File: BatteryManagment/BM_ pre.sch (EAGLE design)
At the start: 2 parts, among them U1 ATMEGA328P-AU

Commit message: Worked at the Schematic
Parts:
- added BATTERY+: Battery+, BM_pre:PAD
- added BATTERY-: PAD, BM_pre:PAD
- added C10, C11, C9: 10u, rcl:C-EUC0805
- added C2, C7: 100n, rcl:C-EUC0603
- added C3, C6: 47u, rcl:C-EUC1812
- added C4, C5: 100u, rcl:CPOL-EUE3.5-10
- added C8: 1u_100V, rcl:C-EUC1206
- added CELL1, CELL2, CELL3, CELL4, CELL5, CELL6, GND, GND14, VIN: TPSQB2,54, testpad:TPSQB2,54
- added L1: 2310-V-RC, BM_pre:2310-V-RC
- added R1: 100k, rcl:R-EU_R0603
- added R10, R11, R12, R13, R2, R3, R4, R5, R6, R7, R8, R9: (no value), rcl:R-EU_R0603
- added U$1, U$3, U$5: SBR10B45P5, BM_pre:SBR10B45P5
- added U$2: IRFS7534-7PPBF, BM_pre:IRFS7534-7PPBF
- added U$4: CRA2512-FZ-R010ELF, BM_pre:CRA2512-FZ-R010ELF
- added U$6: IPB180P04P4L-02, BM_pre:IPB180P04P4L-02
- added U$7: ZXTR2012Z, BM_pre:ZXTR2012Z
- added U$8: NCV78L00A, BM_pre:NCV78L00A
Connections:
- removed net +3V3: C1.1, U1.AVCC, U1.VCC, U1.VCC_2
- new net +12V: C10.1, U$7.VO
- new net +5V: C1.1, C11.1, U$8.VO, U1.AREF, U1.AVCC, U1.VCC, U1.VCC_2
- new net ADC_BAT_1: R2.1, R3.2, U1.PC0
- new net ADC_BAT_2: R4.1, R5.2, U1.PC1
- new net ADC_BAT_3: R6.1, R7.2, U1.PC2
- new net ADC_BAT_4: R11.2, R8.1, U1.PC3
- new net ADC_BAT_5: R12.2, R9.1, U1.PC4
- new net ADC_BAT_6: R10.1, R13.2, U1.PC5
- new net BATTERY+: C9.1, R1.1, U$5.C, U$6.S, U$8.VI
- new net CURRENT+: L1.2, U$4.1
- new net CURRENT-: C5.+, C6.1, C7.1, U$4.2, U$5.A
- new net CURRENTSENSE: U1.ADC6
- new net LOAD_CONTROL: U$2.G
- new net MOTOR+: BATTERY+.TP, U$6.D
- new net MOTOR_CONTROL: R1.2, U$6.G
- new net N$1: C2.1, C3.1, C4.+, U$1.C, U$2.S
- new net N$11: CELL3.TP, R6.2
- new net N$12: CELL4.TP, R8.2
- new net N$13: CELL5.TP, R9.2
- new net N$14: CELL6.TP, R10.2
- new net N$2: L1.1, U$2.D, U$3.C
- new net N$7: CELL1.TP, R2.2
- new net N$8: CELL2.TP, R4.2
- new net VIN_SENSE: C8.1, U$1.A, U$7.VI, U1.ADC7, VIN.TP
- net GND: now also BATTERY-.TP, C10.2, C11.2, C2.2, C3.2, C4.-, C5.-, C6.2, C7.2, C8.2, C9.2, GND.TP, GND14.TP, R11.1, R12.1, R13.1, R3.1, R5.1, R7.1, U$3.A, U$7.GND, U$8.GND
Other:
- note added: "NPN-Transistor"

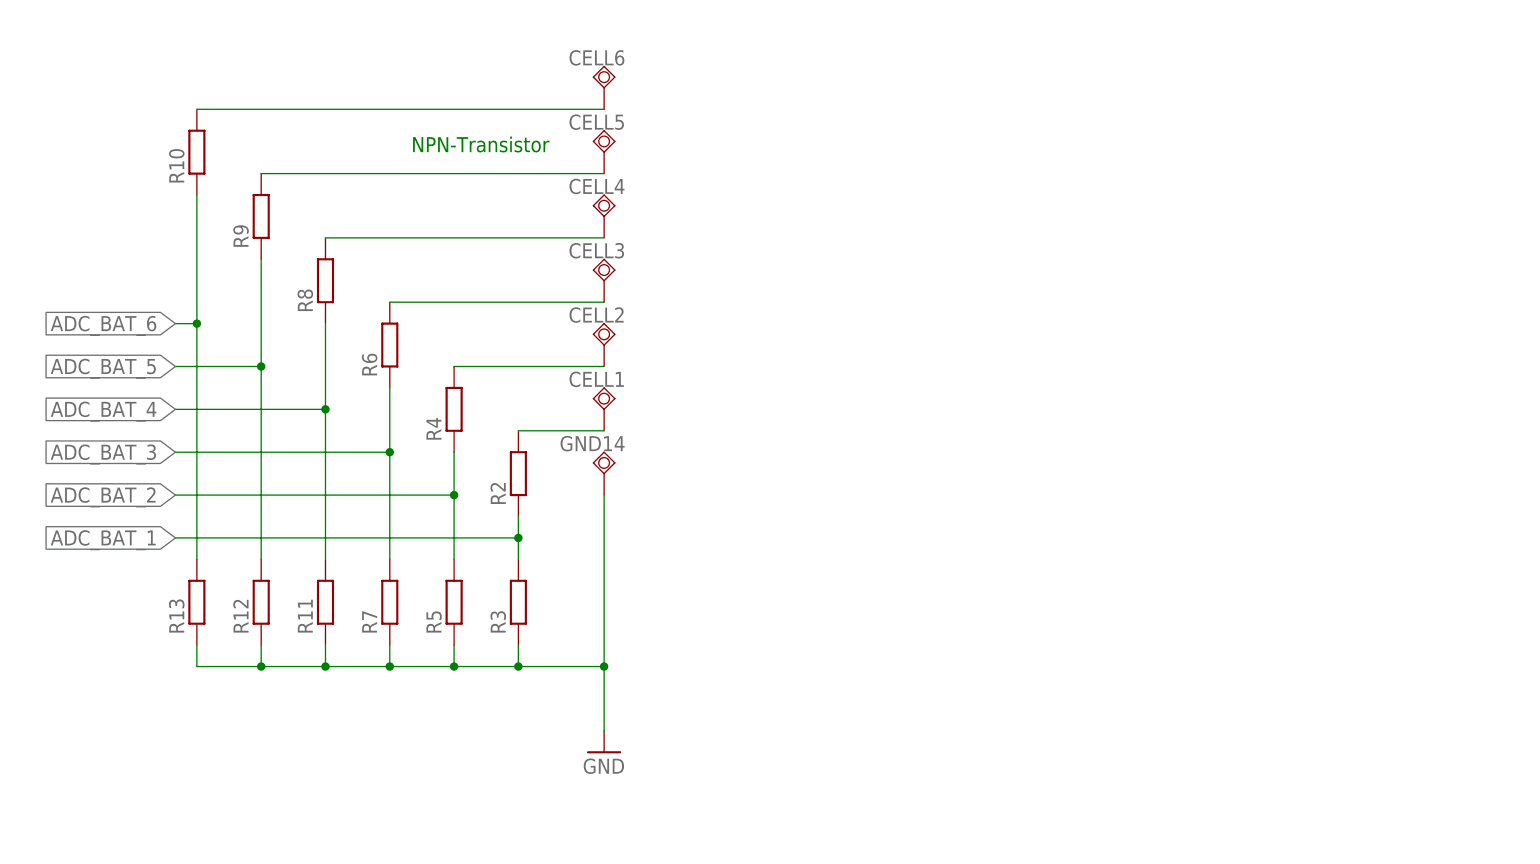
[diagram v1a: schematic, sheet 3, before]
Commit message: Upload it, that i can work at the PC
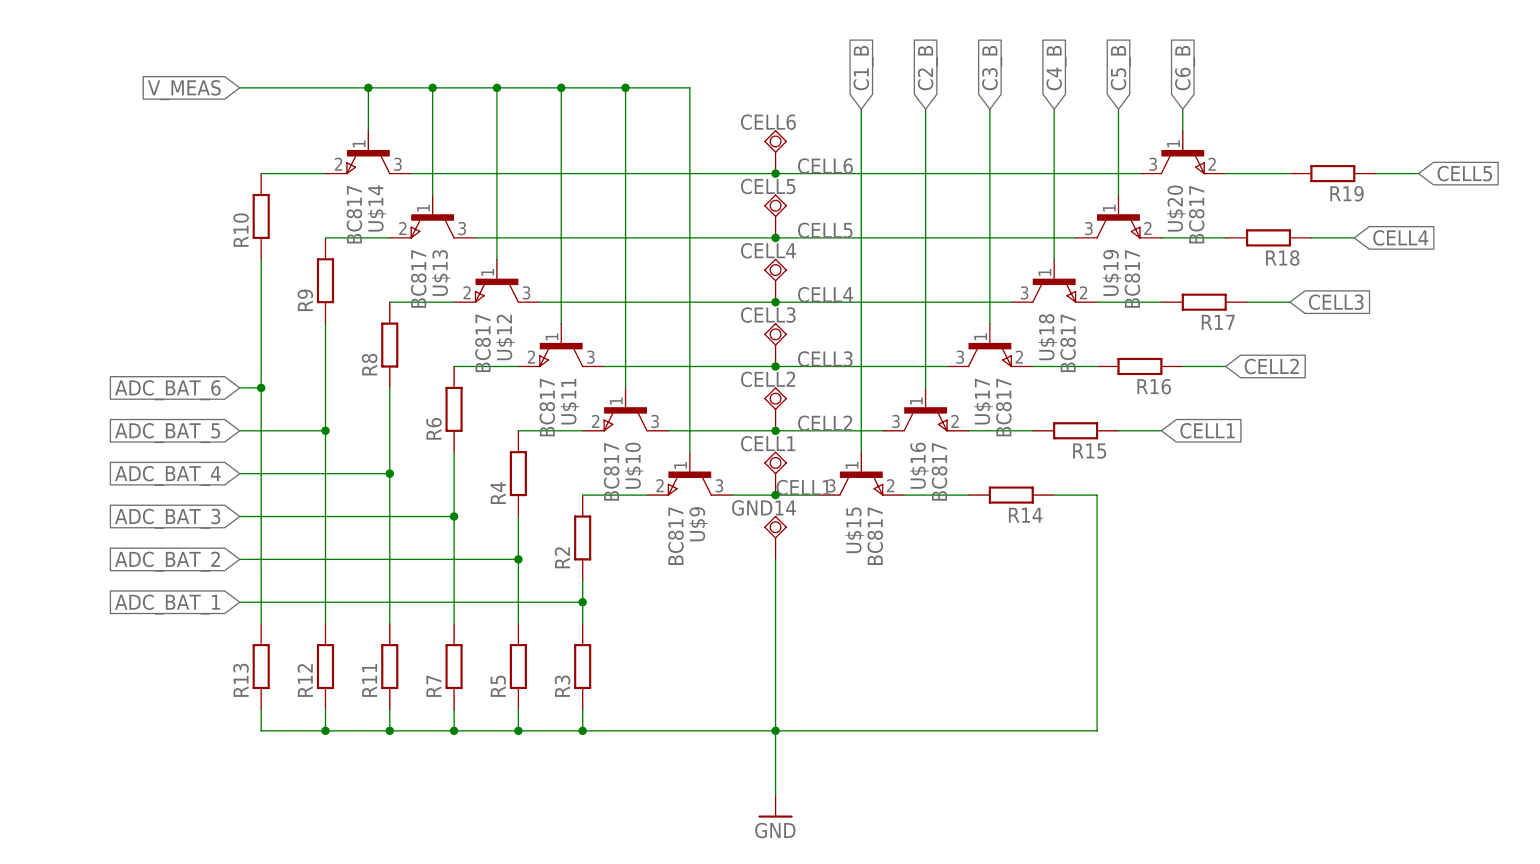
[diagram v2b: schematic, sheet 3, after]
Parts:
- added R14, R15, R16, R17, R18, R19: (no value), rcl:R-EU_R0603
- added U$10, U$11, U$12, U$13, U$14, U$15, U$16, U$17, U$18, U$19, U$20, U$9: BC817, BM_pre:BC817
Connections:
- new net C1_B: U$15.B
- new net C2_B: U$16.B
- new net C3_B: U$17.B
- new net C4_B: U$18.B
- new net C5_B: U$19.B
- new net C6_B: U$20.B
- new net CELL1: CELL1.TP, R15.1, U$15.C, U$9.C
- new net CELL2: CELL2.TP, R16.1, U$10.C, U$16.C
- new net CELL3: CELL3.TP, R17.1, U$11.C, U$17.C
- new net CELL4: CELL4.TP, R18.1, U$12.C, U$18.C
- new net CELL5: CELL5.TP, R19.1, U$13.C, U$19.C
- new net CELL6: CELL6.TP, U$14.C, U$20.C
- new net N$10: R10.2, U$14.E
- new net N$3: R2.2, U$9.E
- new net N$4: R4.2, U$10.E
- new net N$5: R14.2, U$15.E
- new net N$6: R15.2, U$16.E
- new net N$9: R9.2, U$13.E
- new net V_MEAS: U$10.B, U$11.B, U$12.B, U$13.B, U$14.B, U$9.B
- net GND: now also R14.1
- net N$11: now also R16.2, U$17.E; no longer CELL3.TP, R6.2
- net N$12: now also R17.2, U$18.E; no longer CELL4.TP, R8.2
- net N$13: now also R18.2, U$19.E; no longer CELL5.TP, R9.2
- net N$14: now also R19.2, U$20.E; no longer CELL6.TP, R10.2
- net N$7: now also R6.2, U$11.E; no longer CELL1.TP, R2.2
- net N$8: now also R8.2, U$12.E; no longer CELL2.TP, R4.2
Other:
- note removed: "NPN-Transistor"
- moved on the sheet: CELL1, CELL2, CELL3, CELL4, CELL5, CELL6, GND14, R10, R11, R12, R13, R2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
